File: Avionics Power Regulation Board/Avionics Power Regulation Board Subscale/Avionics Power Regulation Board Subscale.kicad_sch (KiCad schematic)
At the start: 7 parts, among them J1 282841-2, J2 282841-2, U1 LM2576HVS-5

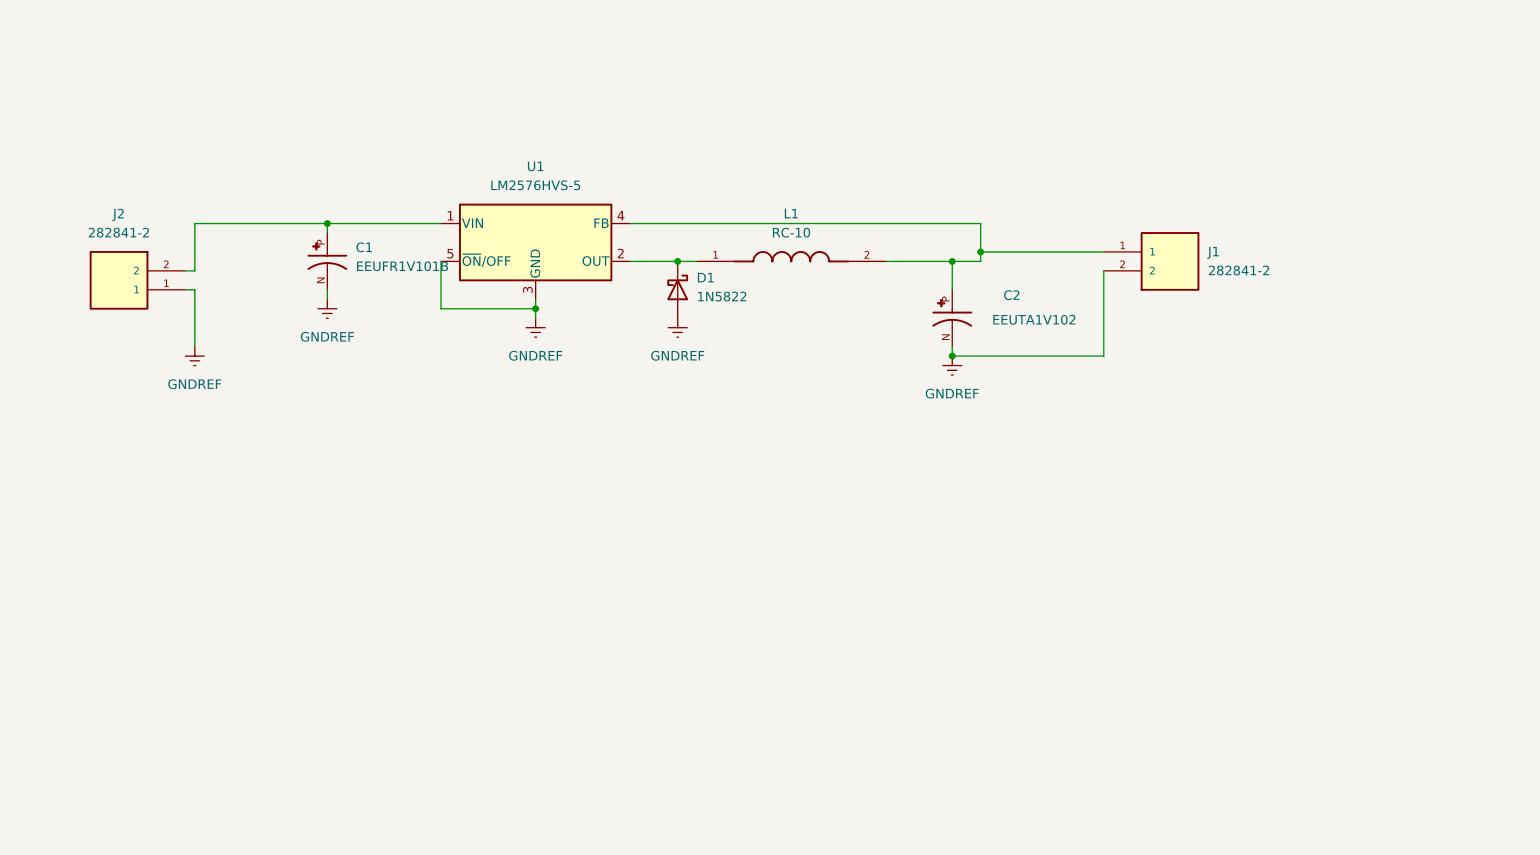
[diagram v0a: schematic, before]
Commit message: Updated Subscale Board
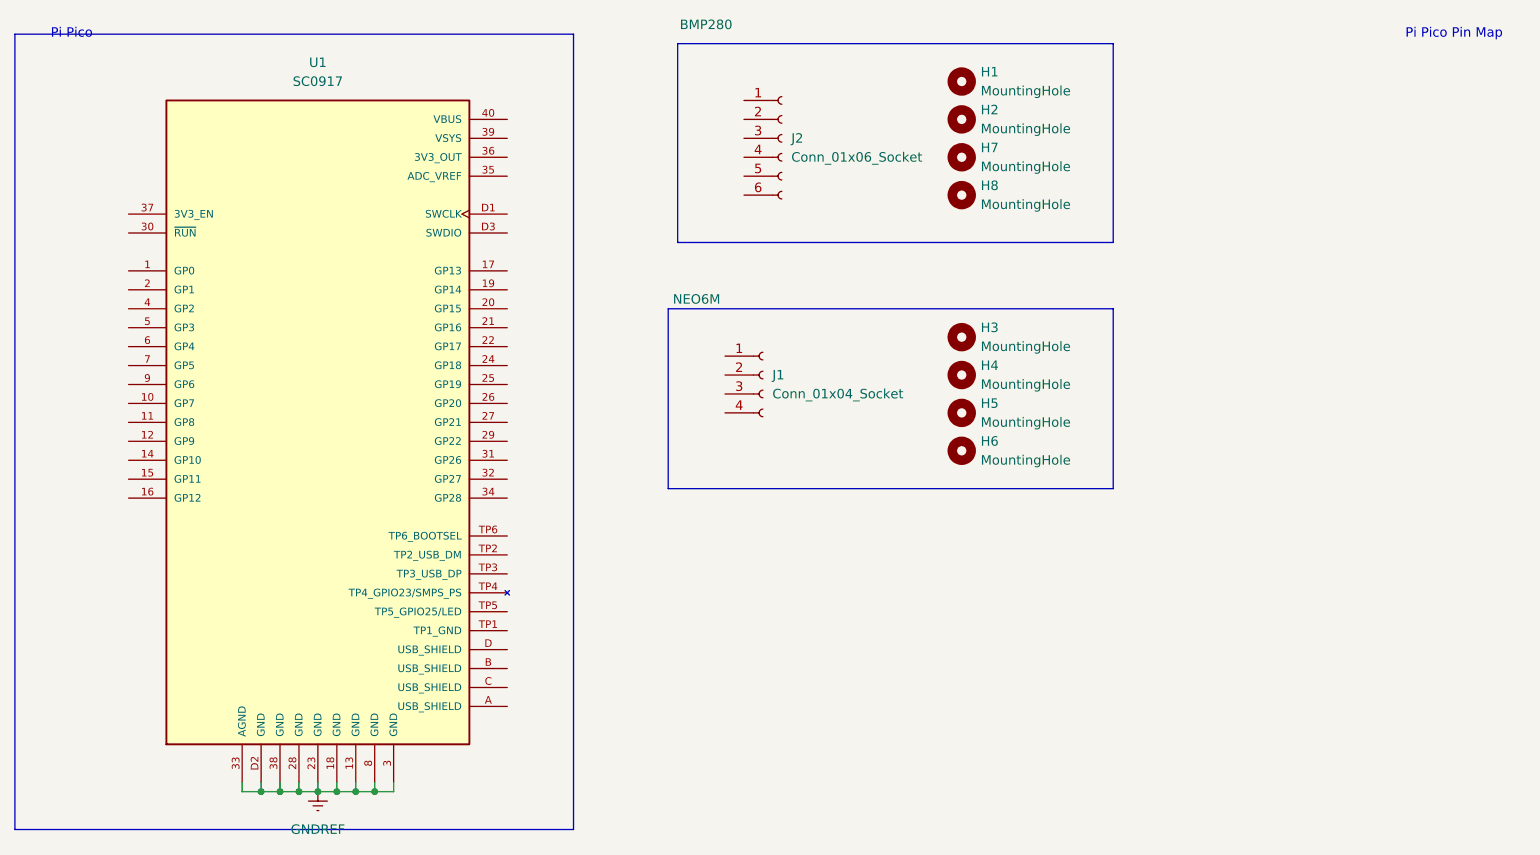
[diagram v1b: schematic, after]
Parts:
- removed C1: EEUFR1V101B, EEUFR1V101B:CAPPRD350W60D800H1150, symbol EEUFR1V101B:EEUFR1V101B
- removed C2: EEUTA1V102, EEUTA1V102:CAPPRD750W80D1600H2500, symbol EEUTA1V102:EEUTA1V102
- removed D1: 1N5822, Diode_THT:D_DO-201AD_P15.24mm_Horizontal, symbol Diode:1N5822
- removed J1, J2: 282841-2, 282841-2:TE_282841-2, symbol 282841-2:282841-2
- removed L1: RC-10, RC-10:IND_RC-10, symbol RC-10:RC-10
- removed U1: LM2576HVS-5, Package_TO_SOT_SMD:TO-263-5_TabPin3, symbol Regulator_Switching:LM2576HVS-5
- added H1, H2, H3, H4, H5, H6, H7, H8: MountingHole, MountingHole:MountingHole_2.1mm, symbol Mechanical:MountingHole
- added J1: Conn_01x04_Socket, Connector_PinSocket_2.54mm:PinSocket_1x04_P2.54mm_Vertical, symbol Connector:Conn_01x04_Socket
- added J2: Conn_01x06_Socket, Connector_PinSocket_2.54mm:PinSocket_1x06_P2.54mm_Vertical, symbol Connector:Conn_01x06_Socket
- added U1: SC0917, SC0917:MODULE_SC0917, symbol SC0917:SC0917
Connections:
- net GNDREF: now also U1.13 (GND), U1.18 (GND), U1.23 (GND), U1.28 (GND), U1.3 (GND), U1.33 (AGND), U1.38 (GND), U1.8 (GND), U1.D2 (GND)
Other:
- note added: "Pi Pico"
- note added: "Pi Pico Pin Map"
